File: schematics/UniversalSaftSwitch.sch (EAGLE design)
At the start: 20 parts, among them IC2 MAX485 CSA, IC3 AT90S2313S, K2 HF115F-024-S3, T1 BC817

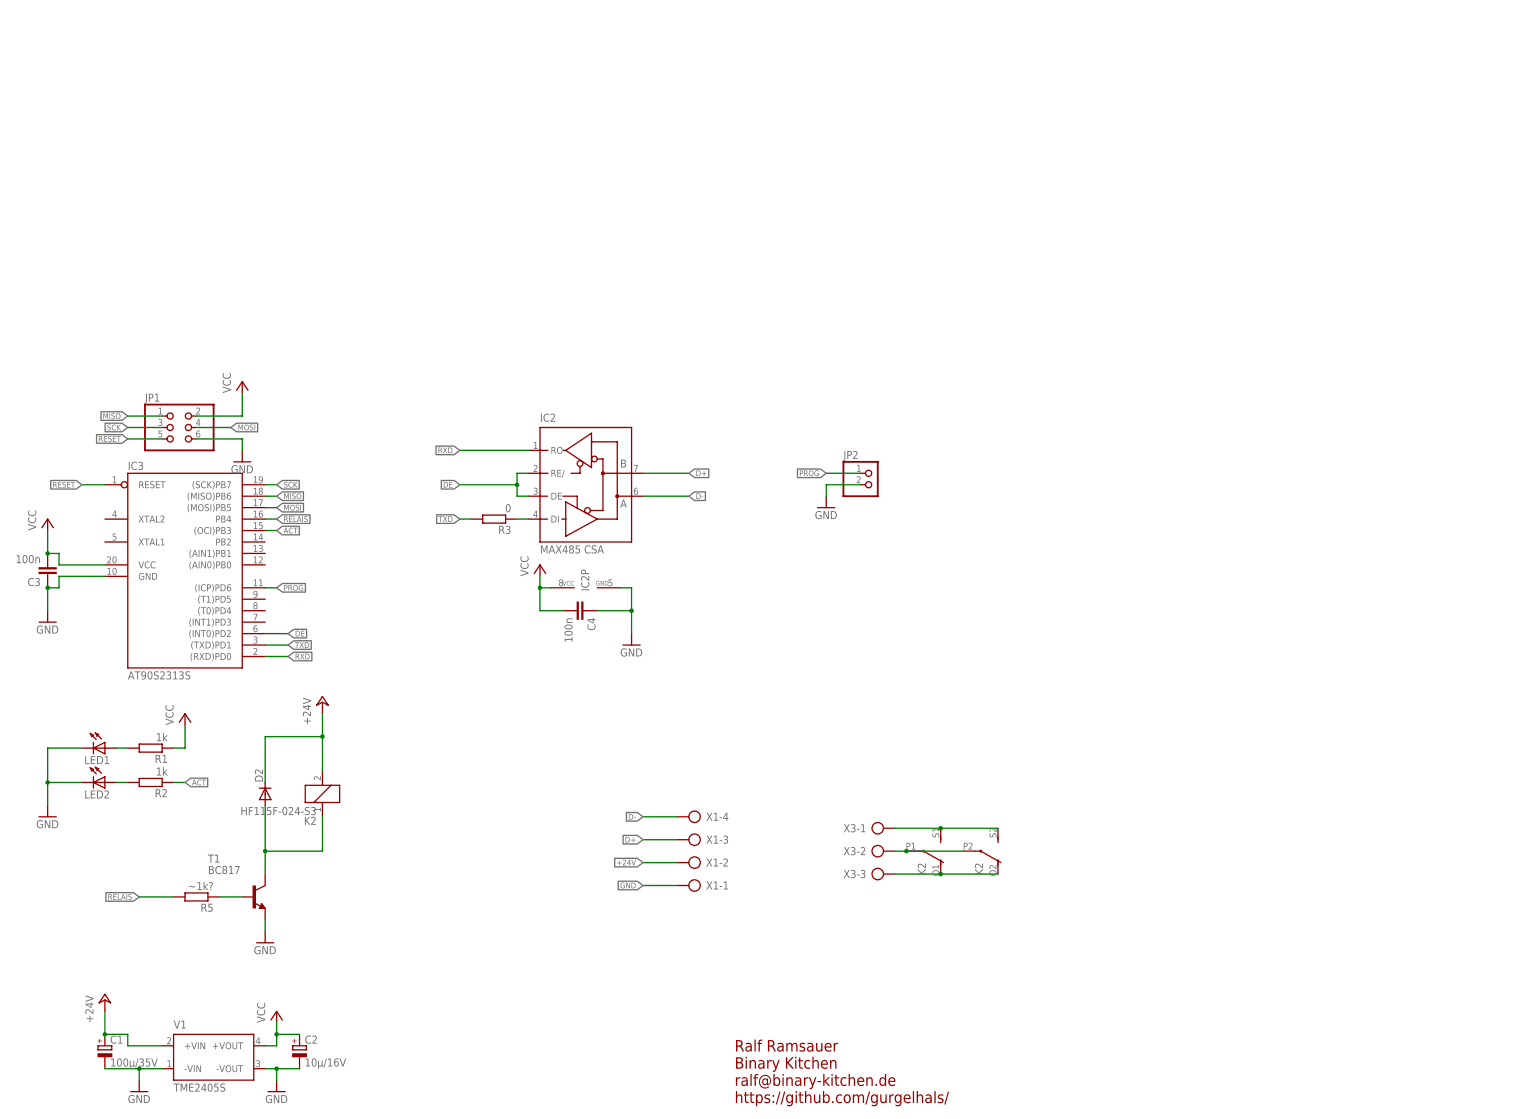
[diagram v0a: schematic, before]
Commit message: New Schematic
Signed-off-by: Ralf Ramsauer <ralf@ramses-pyramidenbau.de>
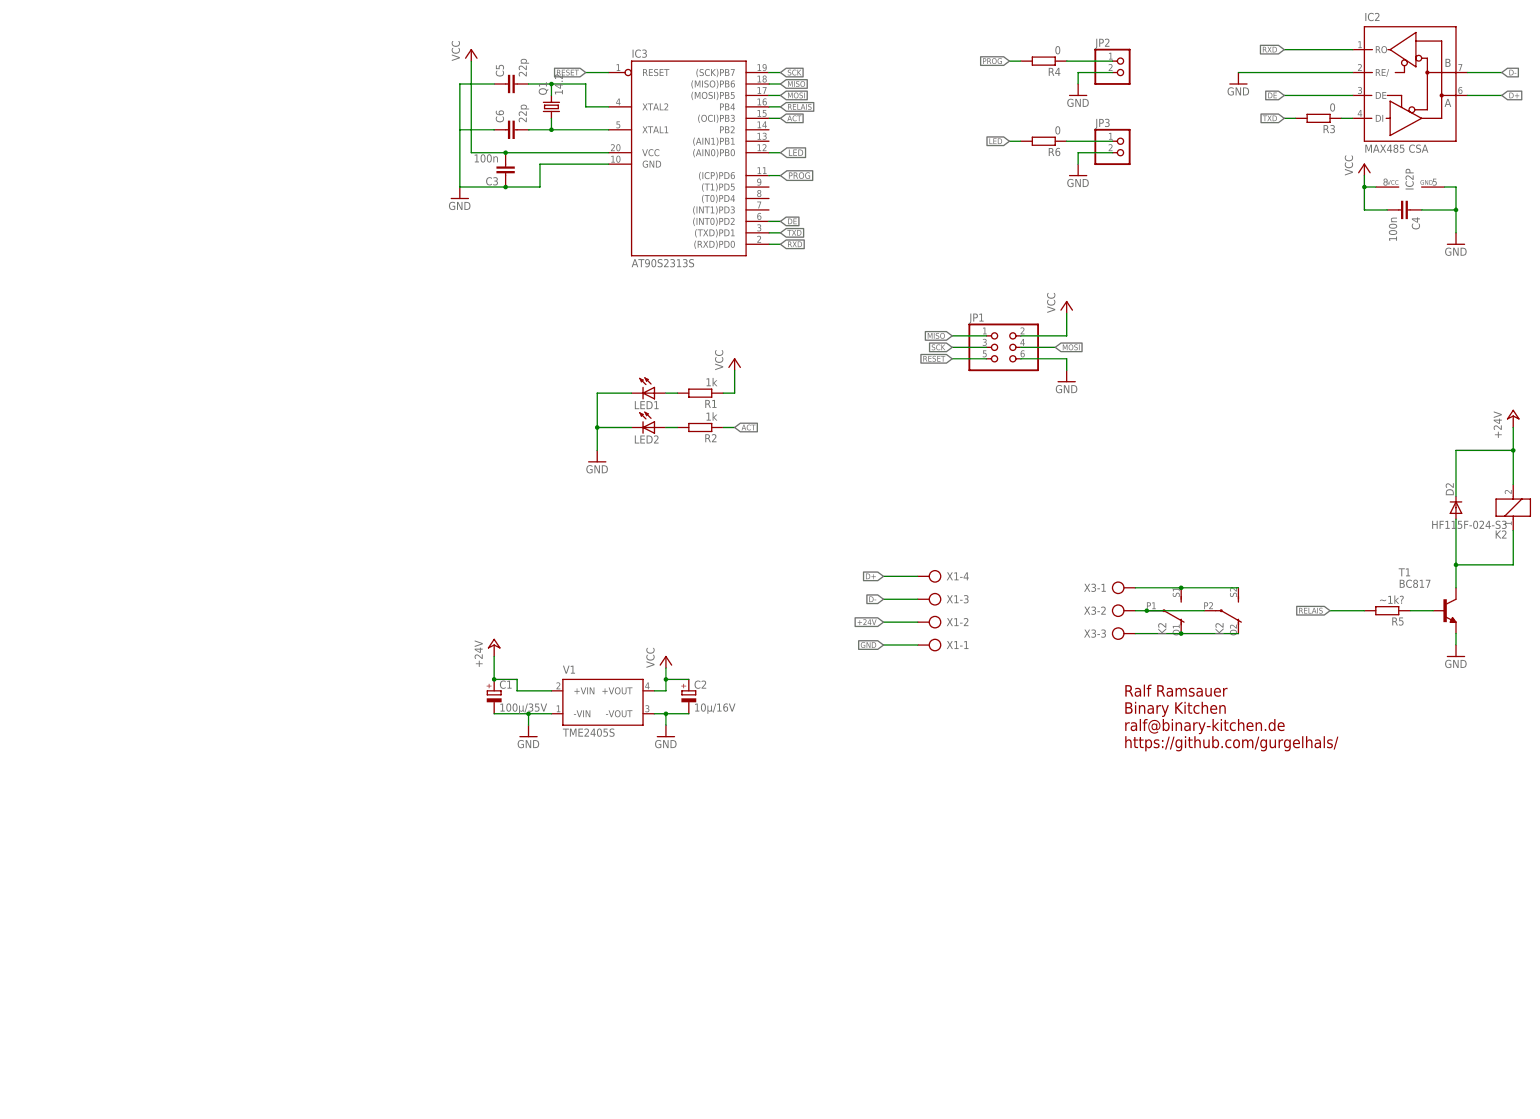
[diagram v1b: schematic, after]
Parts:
- added C5, C6: 22p, rcl:C-EUC0805K
- added JP3: (no value), pinhead:PINHD-1X2
- added Q1: 14.2, crystal:CRYSTALHC49U-V
- added R4, R6: 0, rcl:R-EU_M0805
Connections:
- new net LED: IC3.(AIN0)PB0, R6.2
- new net N$10: C6.2, IC3.XTAL1, Q1.1
- new net N$11: JP2.1, R4.1
- new net N$12: JP3.1, R6.1
- new net N$7: C5.2, IC3.XTAL2, Q1.2
- net D+: now also IC2G$1.A, X1-4.KL; no longer IC2G$1.B, X1-3.KL
- net D-: now also IC2G$1.B, X1-3.KL; no longer IC2G$1.A, X1-4.KL
- net DE: no longer IC2G$1.RE/
- net GND: now also C5.1, C6.1, IC2G$1.RE/, JP3.2
- net PROG: now also R4.2; no longer JP2.1
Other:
- moved on the sheet: C1, C2, C3, C4, D2, IC2, IC2P, IC3, JP1, JP2, K2, LED1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
